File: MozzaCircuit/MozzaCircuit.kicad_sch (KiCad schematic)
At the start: 17 parts, among them J1 8P8C_both_sides, U1 MCP23017_ML, U2 MCP23017_ML_NoTP

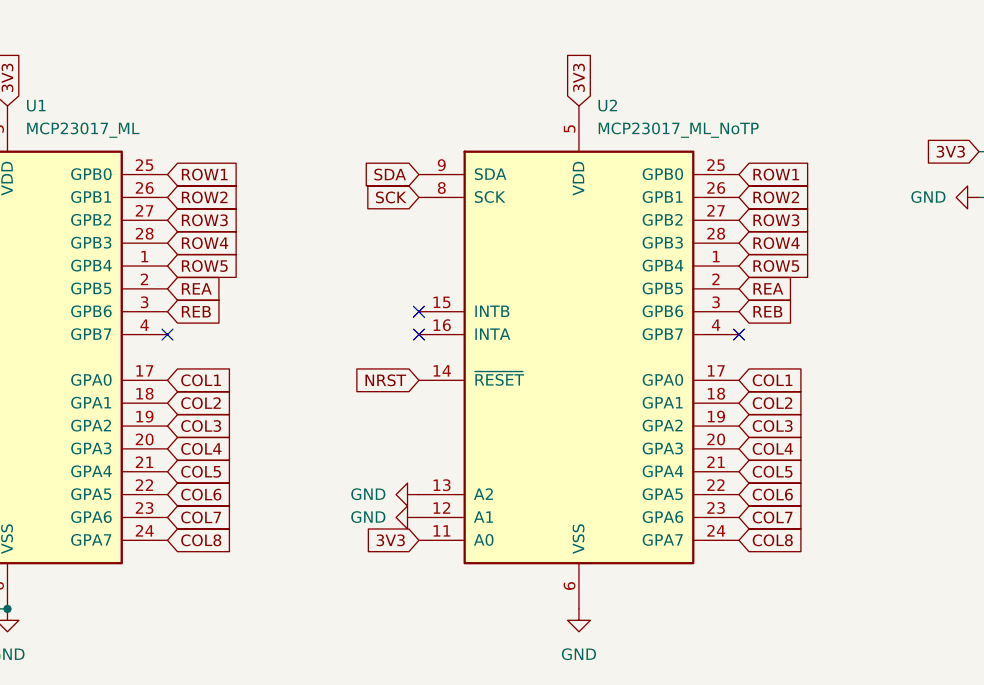
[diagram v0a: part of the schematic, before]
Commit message: expander vias
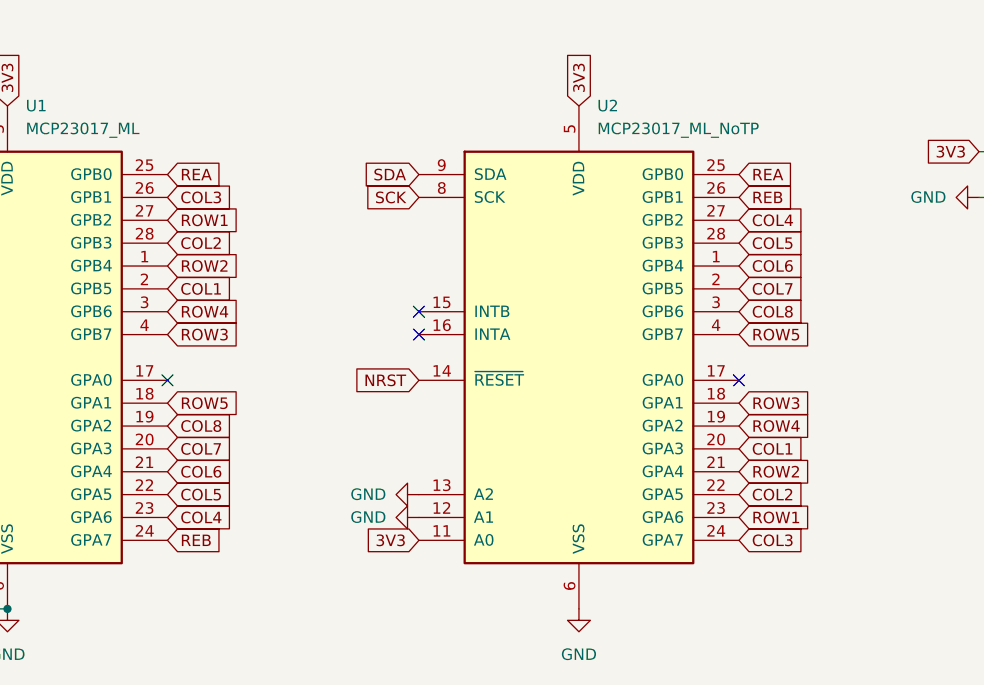
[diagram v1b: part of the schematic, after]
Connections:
- net COL1: now also U1.2 (GPB5), U2.20 (GPA3); no longer U1.17 (GPA0), U2.17 (GPA0)
- net COL2: now also U1.28 (GPB3), U2.22 (GPA5); no longer U1.18 (GPA1), U2.18 (GPA1)
- net COL3: now also U1.26 (GPB1), U2.24 (GPA7); no longer U1.19 (GPA2), U2.19 (GPA2)
- net COL4: now also U1.23 (GPA6), U2.27 (GPB2); no longer U1.20 (GPA3), U2.20 (GPA3)
- net COL5: now also U1.22 (GPA5), U2.28 (GPB3); no longer U1.21 (GPA4), U2.21 (GPA4)
- net COL6: now also U1.21 (GPA4), U2.1 (GPB4); no longer U1.22 (GPA5), U2.22 (GPA5)
- net COL7: now also U1.20 (GPA3), U2.2 (GPB5); no longer U1.23 (GPA6), U2.23 (GPA6)
- net COL8: now also U1.19 (GPA2), U2.3 (GPB6); no longer U1.24 (GPA7), U2.24 (GPA7)
- net REA: now also U1.25 (GPB0), U2.25 (GPB0); no longer U1.2 (GPB5), U2.2 (GPB5)
- net REB: now also U1.24 (GPA7), U2.26 (GPB1); no longer U1.3 (GPB6), U2.3 (GPB6)
- net ROW1: now also U1.27 (GPB2), U2.23 (GPA6); no longer U1.25 (GPB0), U2.25 (GPB0)
- net ROW2: now also U1.1 (GPB4), U2.21 (GPA4); no longer U1.26 (GPB1), U2.26 (GPB1)
- net ROW3: now also U1.4 (GPB7), U2.18 (GPA1); no longer U1.27 (GPB2), U2.27 (GPB2)
- net ROW4: now also U1.3 (GPB6), U2.19 (GPA2); no longer U1.28 (GPB3), U2.28 (GPB3)
- net ROW5: now also U1.18 (GPA1), U2.4 (GPB7); no longer U1.1 (GPB4), U2.1 (GPB4)
